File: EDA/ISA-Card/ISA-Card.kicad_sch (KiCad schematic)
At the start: 26 parts, among them U7101 74HCT245, U7102 74HCT244, U7104 74HCT138, U7105 74HCT138, U7106 74LS08, U7107 74LS32, U7108 74LS32, U7109 74HC368, U7110 74HC04, U7111 74LS125, U7112 74HC74, U7113 74HC74, U7114 74HC4024, U7115 74HC4024, U7116 74HC595, U7117 74HC595, U7118 74HC595, U7119 8251, U7120 26LS31, U7121 26LS32, X3 DB15_Female, X5 Conn_02x08_Counter_Clockwise

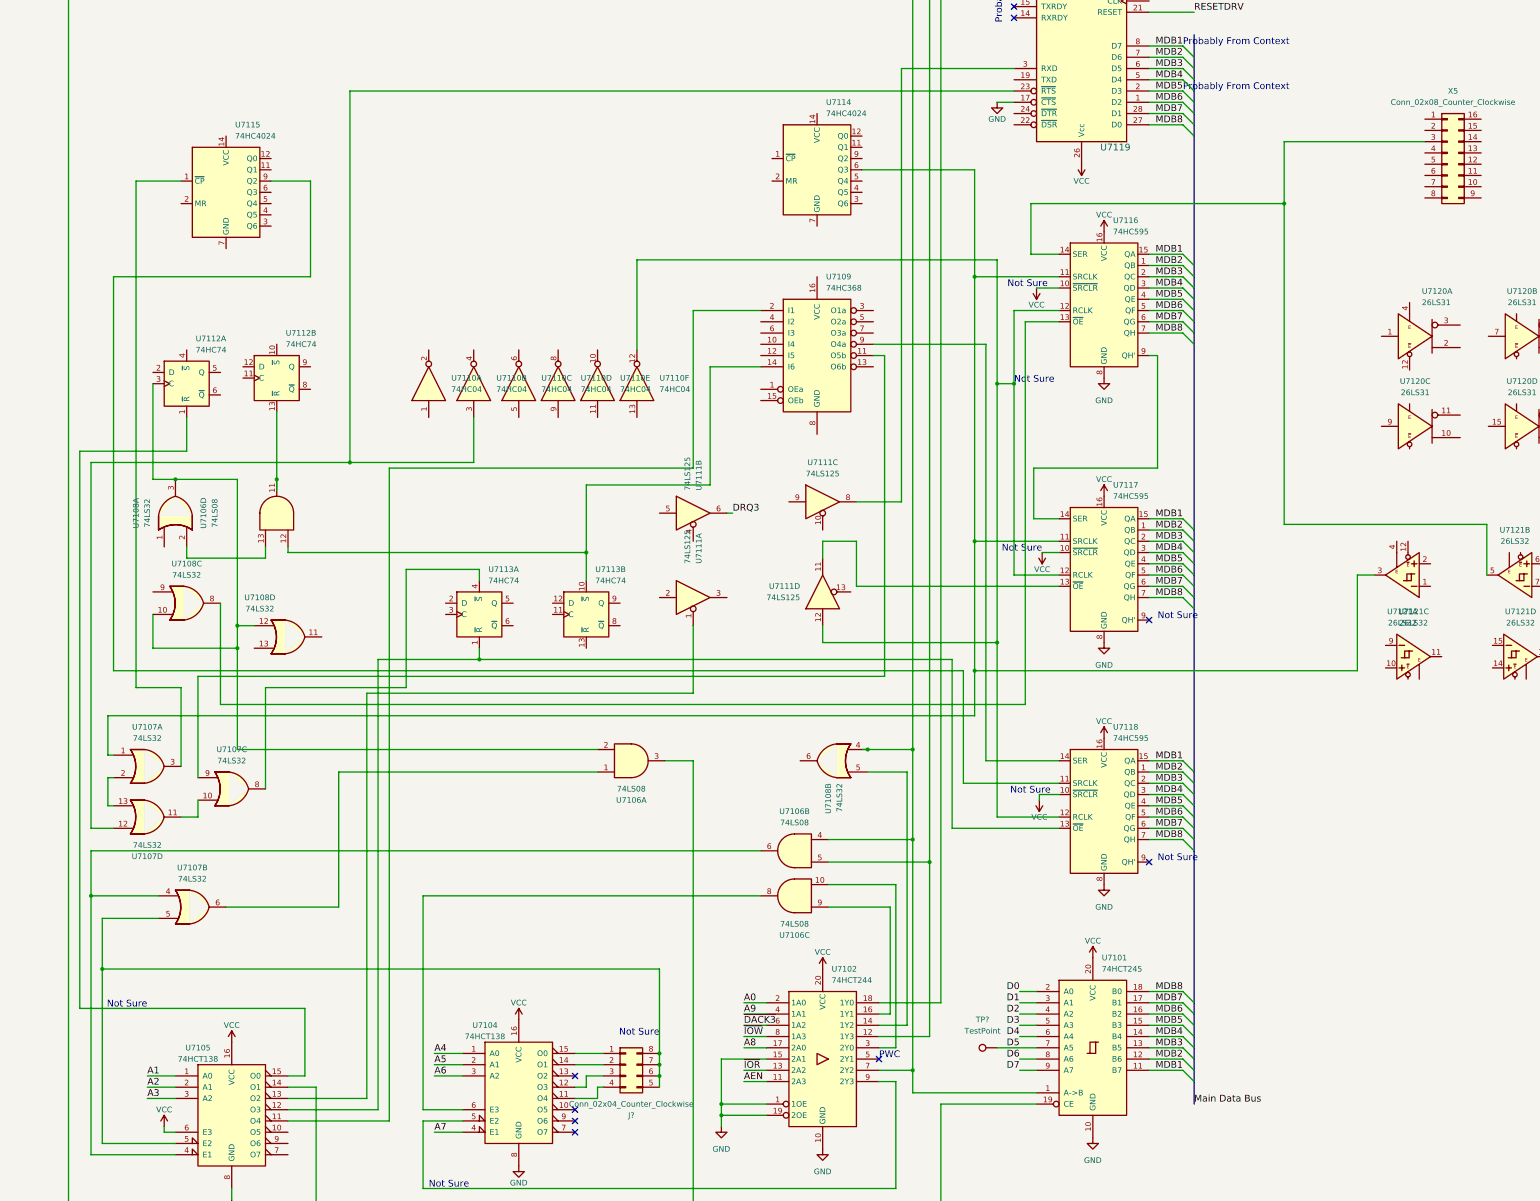
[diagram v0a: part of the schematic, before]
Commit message: 1711 finished
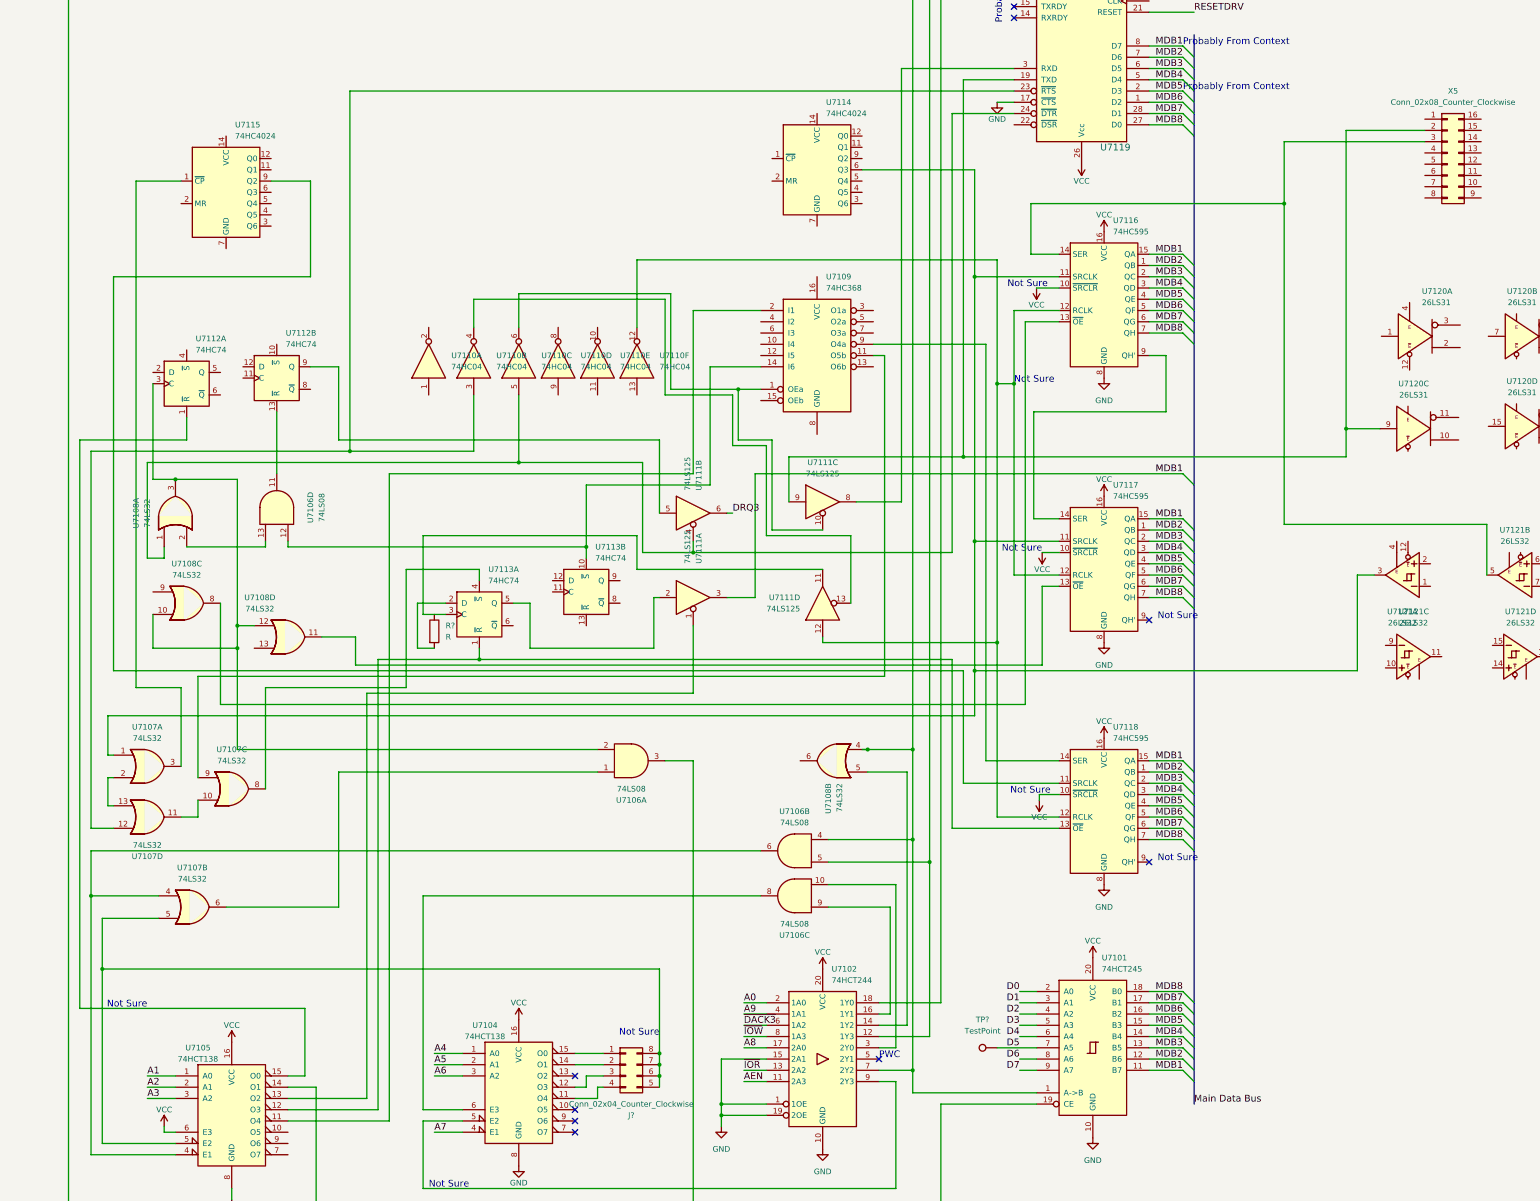
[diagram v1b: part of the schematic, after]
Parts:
- added R?: R, symbol Device:R
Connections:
- net MDB1: now also U7111.3
- net at X5.2 (Pin_2): now also U7111.9, U7119.19 (TXD), U7120.9
- net at U7110.5: now also U7108.1, U7111.4, U7119.24 (~{DTR})
- net at U7110.6: now also U7109.1 (OEa), U7111.10
- net at U7110.4: now also U7111.13
- net at U7111.5: now also U7112.9 (Q)
- net at U7111.2: now also U7113.5 (Q)
- net at U7111.11: now also U7113.3 (C); no longer U7117.13 (~{OE})
- net at U7108.11: now also U7117.13 (~{OE})
- net at U7113.2 (D): now also R?.2
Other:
- moved on the sheet: U7106D, U7110A, U7110B, U7110C, U7110D, U7110E, U7110F, U7111D, U7113B, U7120C
